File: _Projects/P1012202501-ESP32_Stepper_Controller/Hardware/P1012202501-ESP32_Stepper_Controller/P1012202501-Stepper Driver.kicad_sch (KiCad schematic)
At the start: 1 part, among them CN6 KPTBP04R1-500-04BE

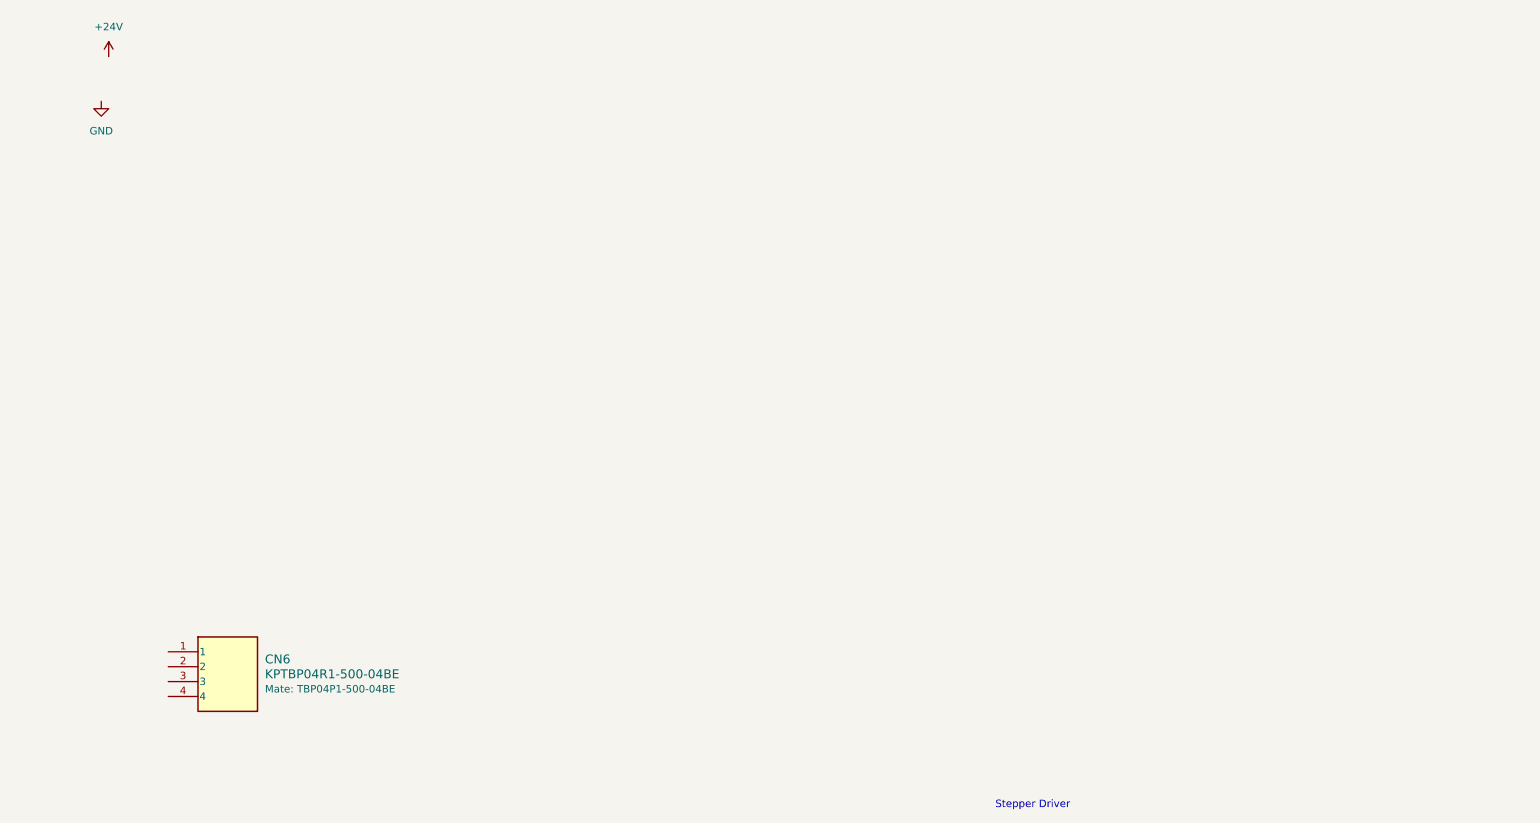
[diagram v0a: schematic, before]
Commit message: Added new content from recent stream.
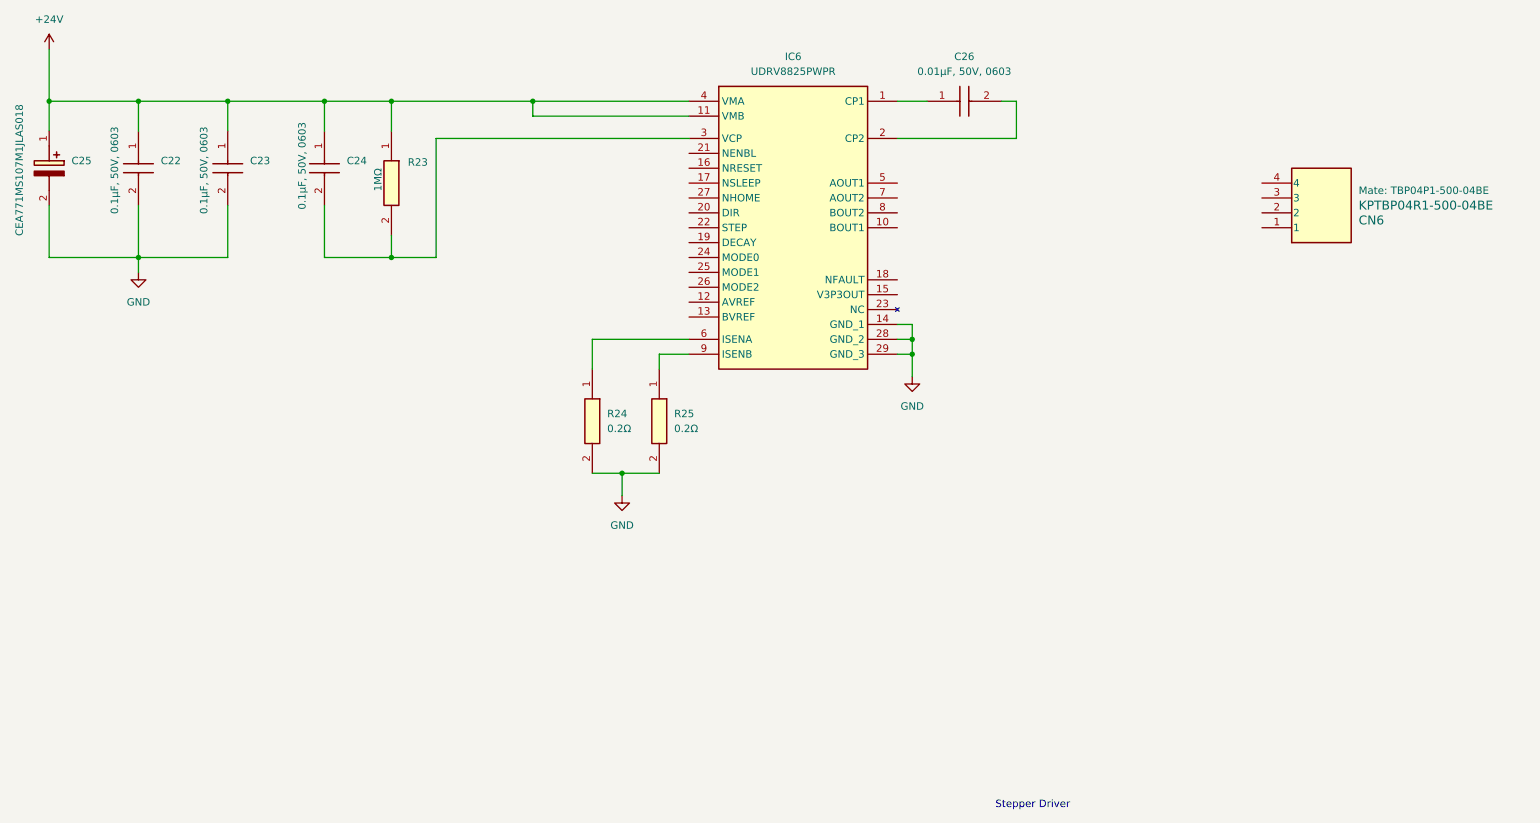
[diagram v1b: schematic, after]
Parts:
- added C22, C23, C24: CC0603104050AAAX7R, COMPONENTS:CAP-0603, symbol COMPONENTS:CC0603104050AAAX7R
- added C25: CEA771MS107M1JLAS018, COMPONENTS:A768MS157M1HLAE024, symbol COMPONENTS:CEA771MS107M1JLAS018
- added C26: CC0603103050AAAX7R, COMPONENTS:CAP-0603, symbol COMPONENTS:CC0603103050AAAX7R
- added IC6: UDRV8825PWPR, COMPONENTS:HTSSOP-28, symbol COMPONENTS:UDRV8825PWPR
- added R23: RC06031M0075AAA, COMPONENTS:RES-0603, symbol COMPONENTS:RC06031M0075AAA
- added R24, R25: RC08050R2075AAE, COMPONENTS:RES-0805, symbol COMPONENTS:RC08050R2075AAE
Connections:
- net +24V: now also C22.1, C23.1, C24.1, C25.1 (+), IC6.11 (VMB), IC6.4 (VMA), R23.1
- net GND: now also C22.2, C23.2, C25.2 (-), IC6.14 (GND_1), IC6.28 (GND_2), IC6.29 (GND_3), R24.2, R25.2
- new net: IC6.9 (ISENB), R25.1
- new net: C26.1, IC6.1 (CP1)
- new net: C26.2, IC6.2 (CP2)
- new net: IC6.6 (ISENA), R24.1
- new net: C24.2, IC6.3 (VCP), R23.2
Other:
- moved on the sheet: CN6

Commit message: Adding new materials from stream.
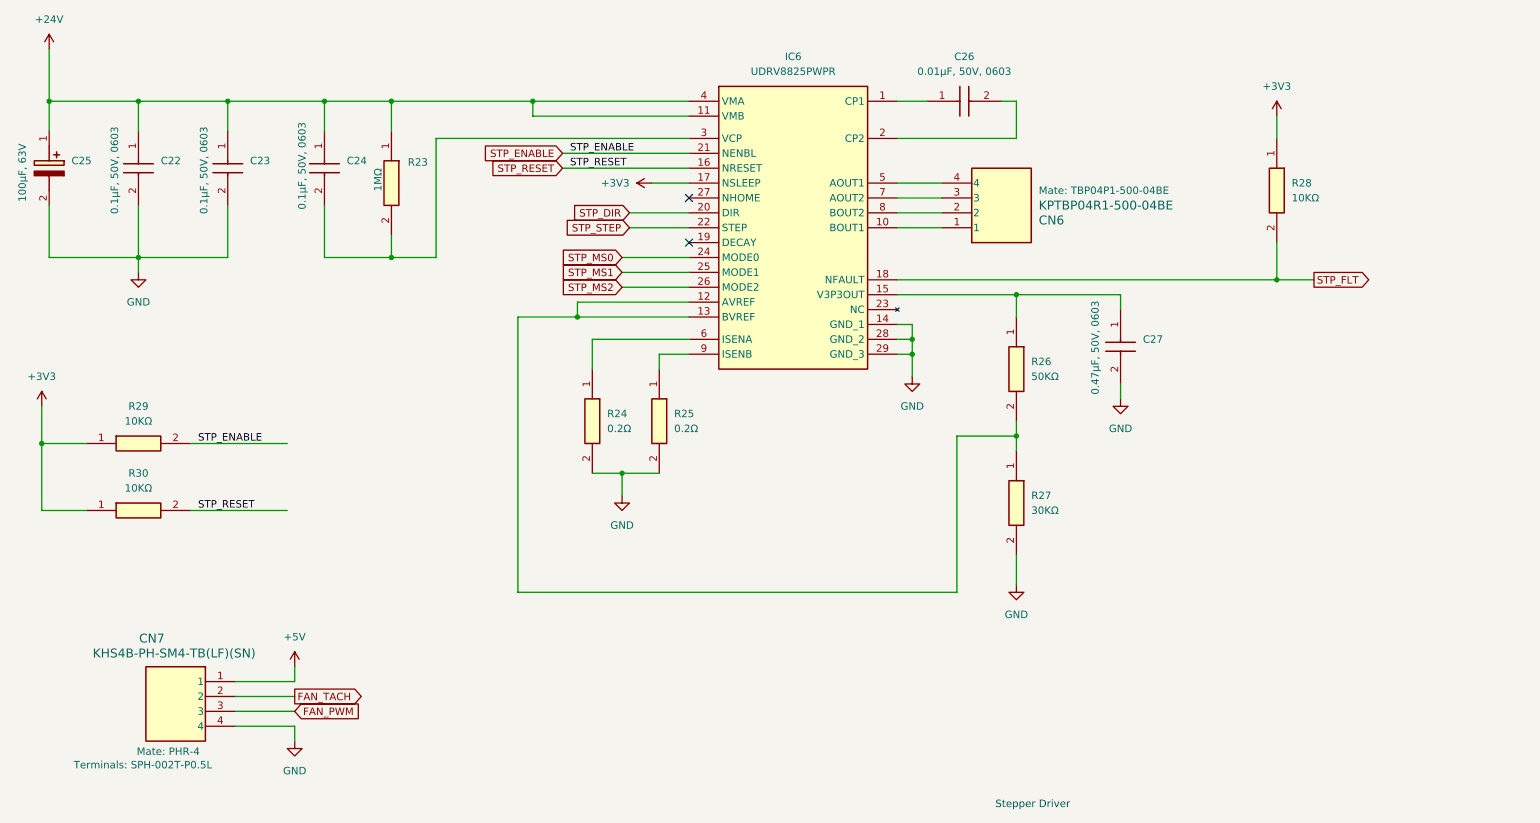
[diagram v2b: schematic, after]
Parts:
- added C27: CC0603474050AAAX7R, COMPONENTS:CAP-0603, symbol COMPONENTS:CC0603474050AAAX7R
- added CN7: KHS4B-PH-SM4-TB(LF)(SN), CONNECTORS:S4B-PH-SM4-TB, symbol CONNECTORS:KHS4B-PH-SM4-TB(LF)(SN)
- added R26: RC060350K075AAA, COMPONENTS:RES-0603, symbol COMPONENTS:RC060350K075AAA
- added R27: RC060330K075AAA, COMPONENTS:RES-0603, symbol COMPONENTS:RC060330K075AAA
- added R28, R29, R30: RC060310K2075AAA, COMPONENTS:RES-0603, symbol COMPONENTS:RC060310K2075AAA
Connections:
- net GND: now also C27.2, CN7.4, R27.2
- net at CN6.1: now also IC6.10 (BOUT1)
- net at CN6.2: now also IC6.8 (BOUT2)
- net at CN6.3: now also IC6.7 (AOUT2)
- net at CN6.4: now also IC6.5 (AOUT1)
- net at IC6.12 (AVREF): now also IC6.13 (BVREF), R26.2, R27.1
- net at IC6.15 (V3P3OUT): now also C27.1, R26.1
- net STP_RESET: now reaches IC6.16 (NRESET)
- net STP_RESET: now also R30.2
- net +3V3: now reaches IC6.17 (NSLEEP)
- net +3V3: now also R28.1, R29.1, R30.1
- net STP_FLT: now reaches IC6.18 (NFAULT)
- net STP_FLT: now also R28.2
- net STP_DIR: now reaches IC6.20 (DIR)
- net STP_ENABLE: now reaches IC6.21 (NENBL)
- net STP_ENABLE: now also R29.2
- net STP_STEP: now reaches IC6.22 (STEP)
- net STP_MS0: now reaches IC6.24 (MODE0)
- net STP_MS1: now reaches IC6.25 (MODE1)
- net STP_MS2: now reaches IC6.26 (MODE2)
- new net +5V: CN7.1
- new net FAN_PWM: CN7.3
- new net FAN_TACH: CN7.2
- no-connect marks 0 -> 2
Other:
- moved on the sheet: CN6
